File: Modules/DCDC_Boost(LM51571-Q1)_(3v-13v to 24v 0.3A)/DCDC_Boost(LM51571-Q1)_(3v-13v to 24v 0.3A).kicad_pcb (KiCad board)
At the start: 2 copper layers, 1 part, among them U1 LM51571

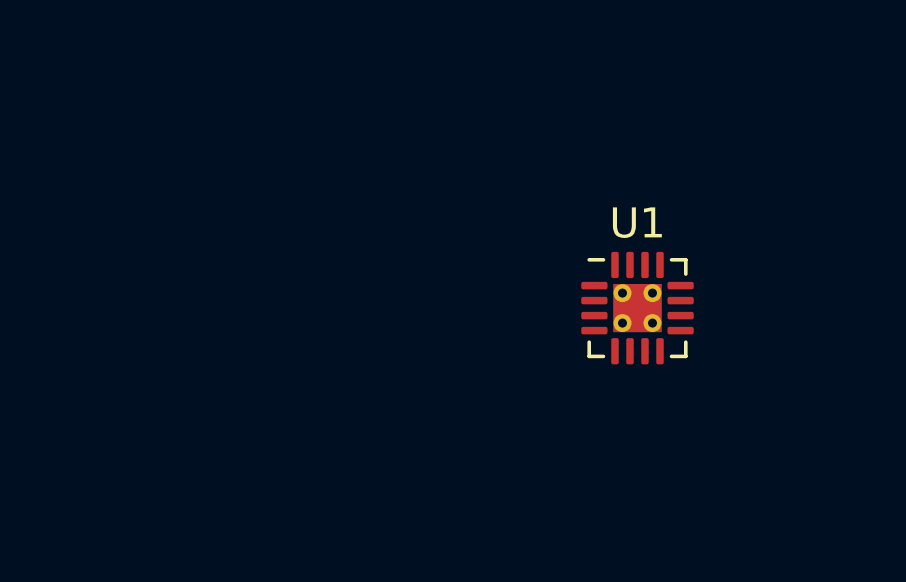
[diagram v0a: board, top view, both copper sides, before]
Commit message: update modules
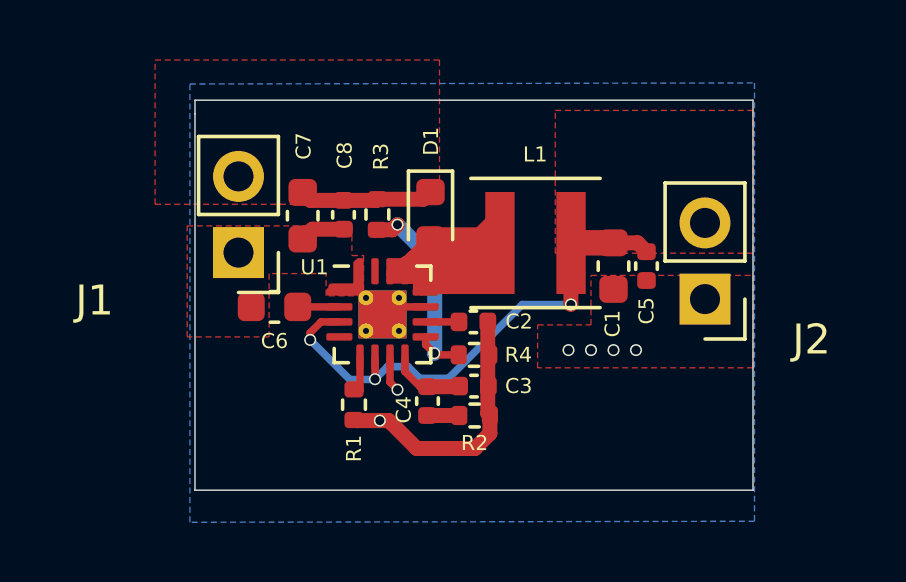
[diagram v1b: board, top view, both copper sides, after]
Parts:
- added C1: 4.7uF, Capacitor_SMD:C_0603_1608Metric, F.Cu at (128.0, 69.7)
- added C2: 68nF, Capacitor_SMD:C_0402_1005Metric, F.Cu at (123.3, 71.6)
- added C3: 300pF, Capacitor_SMD:C_0402_1005Metric, F.Cu at (123.3, 73.7)
- added C4: 27nF, Capacitor_SMD:C_0402_1005Metric, F.Cu at (121.8, 74.2)
- added C5: 100nF, Capacitor_SMD:C_0402_1005Metric, F.Cu at (129.1, 69.7)
- added C6: 1uF, Capacitor_SMD:C_0603_1608Metric, F.Cu at (116.7, 71.1)
- added C7: 4.7uF, Capacitor_SMD:C_0603_1608Metric, F.Cu at (117.6, 68.0)
- added C8: 100nF, Capacitor_SMD:C_0402_1005Metric, F.Cu at (119.0, 68.0)
- added D1: 0.55V 1A, Diode_SMD:D_0603_1608Metric, F.Cu at (121.9, 68.0)
- added J1: Conn_01x02, Connector_PinHeader_2.54mm:PinHeader_1x02_P2.54mm_Vertical, F.Cu at (115.5, 69.2)
- added J2: Conn_01x02, Connector_PinHeader_2.54mm:PinHeader_1x02_P2.54mm_Vertical, F.Cu at (131.1, 70.8)
- added L1: 8.2uH, Inductor_SMD:L_Coilcraft_XxL4020, F.Cu at (125.4, 68.9)
- added R1: 24.9K, Resistor_SMD:R_0402_1005Metric, F.Cu at (119.3, 74.3)
- added R2: 1.18K, Resistor_SMD:R_0402_1005Metric, F.Cu at (123.4, 74.7)
- added R3: 57.6K, Resistor_SMD:R_0402_1005Metric, F.Cu at (120.1, 68.0)
- added R4: 2.49K, Resistor_SMD:R_0402_1005Metric, F.Cu at (123.3, 72.7)
- U1: footprint Package_CSP:LFCSP-16-1EP_3x3mm_P0.5mm_EP1.6x1.6mm_ThermalVias -> Package_DFN_QFN:WQFN-16-1EP_3x3mm_P0.5mm_EP1.6x1.6mm_ThermalVias
- moved U1 8.50 mm to (120.3, 71.3)
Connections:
- U1 pad 1: Net-(U1-Pad1) -> GND
- U1 pad 11: Net-(U1-Pad11) -> GND
- U1 pad 12: Net-(U1-Pad12) -> Net-(D1-Pad2)
- U1 pad 13: Net-(U1-Pad13) -> Net-(D1-Pad2)
- U1 pad 14: Net-(U1-Pad14) -> Net-(D1-Pad2)
- U1 pad 15: Net-(U1-Pad15) -> (no net)
- U1 pad 16: Net-(U1-Pad16) -> GND
- U1 pad 17: Net-(U1-Pad17) -> GND
- U1 pad 3: Net-(U1-Pad3) -> BAT
- U1 pad 4: Net-(U1-Pad4) -> (no net)
- U1 pad 6: Net-(U1-Pad6) -> BAT
- U1 pad 7: Net-(U1-Pad7) -> GND
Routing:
- net BAT: track 0.00 -> 20.2 mm, vias 0 -> 3
- net Net-(D1-Pad2): track 0.00 -> 18.2 mm
- net GND: track 0.00 -> 17.3 mm, vias 0 -> 6
- net V24: track 0.00 -> 7.07 mm
- net Net-(R3-Pad2): track 0.00 -> 7.05 mm, vias 0 -> 2
- net Net-(C3-Pad1): track 0.00 -> 2.51 mm
- net Net-(C6-Pad2): track 0.00 -> 1.39 mm
- net Net-(R1-Pad1): track 0.00 -> 1.21 mm
- net Net-(C2-Pad1): track 0.00 -> 1.17 mm
- net Net-(C4-Pad2): track 0.00 -> 1.06 mm
- added copper zone on F.Cu, net BAT
- added copper zone on B.Cu, net GND
- added copper zone on F.Cu, net GND
- added copper zone on F.Cu, net V24
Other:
- board outline added: 18.6 x 13 mm
- net class Default: clearance 0.2 -> 0.15; trace_width 0.25 -> 0.2; via_dia 0.8 -> 0.4; via_drill 0.4 -> 0.3
- rule trace_clearance: 0.2 -> 0.15
